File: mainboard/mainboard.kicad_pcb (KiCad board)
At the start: 2 copper layers, 50 x 99.1 mm, 93 parts, among them J1 Eurorack_Power, J2 Inv1, J3 Inv2, J4 Ver2, J5 Ver1, J6 Conn_02x04_Counter_Clockwise, J7 Conn_02x03_Counter_Clockwise, J8 Out2, J9 Out1, Q1 BC557, Q10 BC557, Q11 BC557, Q12 BC557, Q13 BC547, Q14 BC547, Q15 BC557, Q16 BC557, Q17 BC547, Q18 BC547, Q19 BC557, Q2 BC557, Q20 BC557, Q21 BC547, Q22 BC547, Q23 BC557, Q24 BC547, Q25 BC547, Q3 BC547, Q4 BC547, Q5 BC547, Q6 BC547, Q7 BC547, Q8 BC547, Q9 BC557, U1 L78L09_TO92, U2 TL074

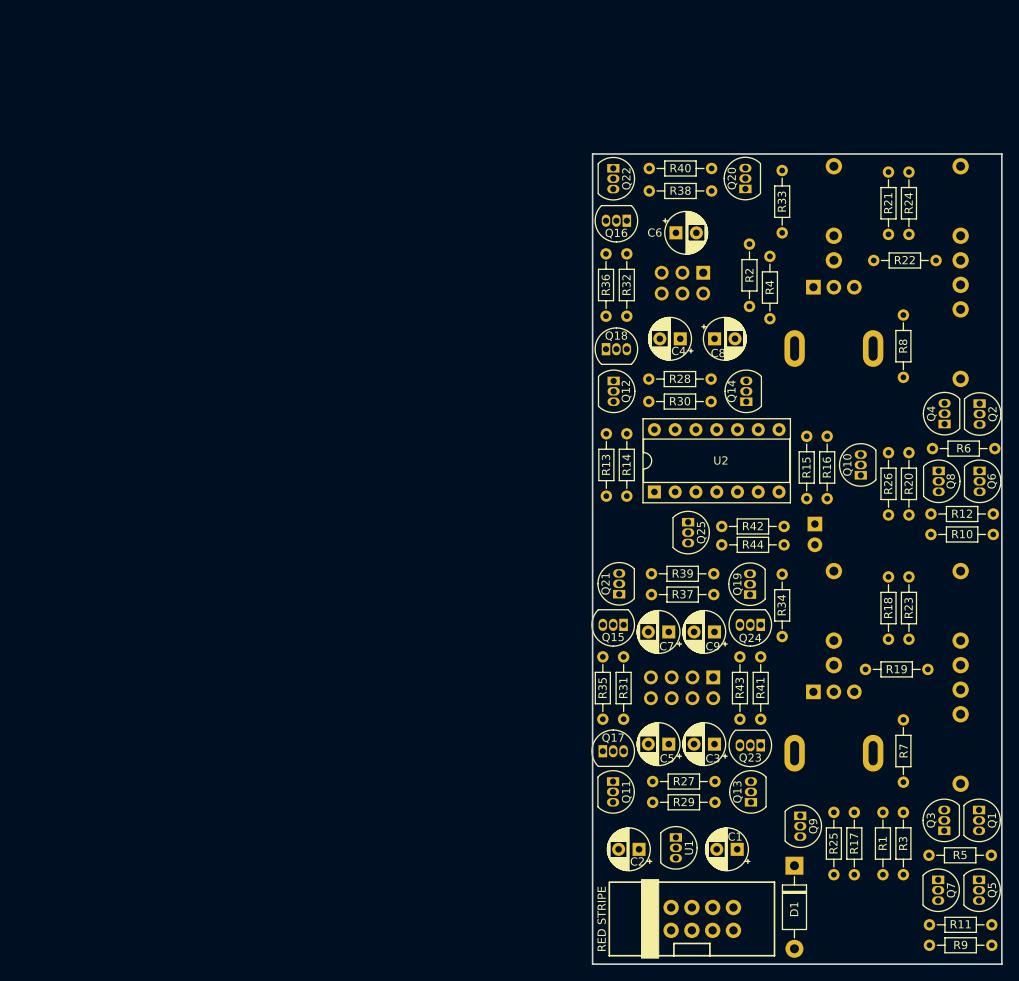
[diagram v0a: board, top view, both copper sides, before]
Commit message: Routing
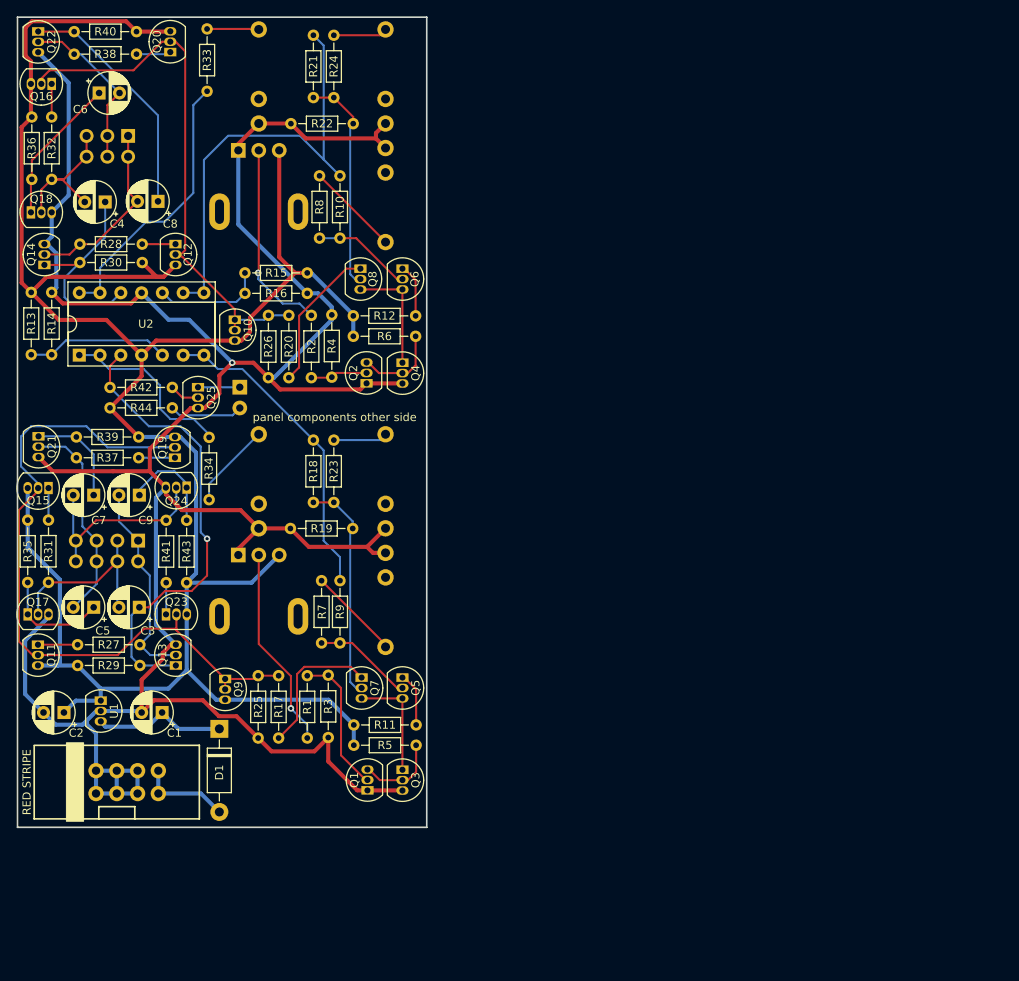
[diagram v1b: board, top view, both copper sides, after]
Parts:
- moved Q14 87.4 mm to (16.8, 44.0)
- moved R9 84.8 mm to (52.9, 82.7), turned to -90 degrees
- moved R10 84.5 mm to (52.9, 33.1), turned to -90 degrees
- moved R30 79.0 mm to (21.1, 43.8), turned to 0 degrees
- moved R28 78.9 mm to (21.1, 41.5), turned to 0 degrees
- moved Q10 78.9 mm to (40.1, 50.8), turned to -90 degrees
- moved R44 76.7 mm to (24.8, 61.5)
- moved R20 76.4 mm to (46.7, 57.8), turned to 90 degrees
- moved R26 76.4 mm to (44.2, 57.8), turned to 90 degrees
- moved R16 75.5 mm to (41.3, 47.5), turned to 0 degrees
- moved Q2 75.0 mm to (56.2, 58.5), turned to 90 degrees
- moved Q8 74.9 mm to (55.4, 44.5)
- moved Q1 74.8 mm to (56.3, 108.3), turned to 90 degrees
- moved Q6 74.8 mm to (60.6, 44.5)
- moved Q5 74.7 mm to (60.6, 94.5)
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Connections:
- U2 pad 1: MIDO1 -> Net-(R34-Pad2)
- U2 pad 10: Net-(C4-Pad1) -> Net-(R15-Pad2)
- U2 pad 12: Net-(R15-Pad2) -> Net-(C4-Pad1)
- U2 pad 13: MIDO2 -> Net-(R33-Pad2)
- U2 pad 14: MIDO2 -> Net-(R33-Pad2)
- U2 pad 2: MIDO1 -> Net-(R34-Pad2)
- U2 pad 3: Net-(R13-Pad2) -> Out1
- U2 pad 5: Out1 -> Net-(R13-Pad2)
- U2 pad 6: Net-(R34-Pad2) -> MIDO1
- U2 pad 7: Net-(R34-Pad2) -> MIDO1
- U2 pad 8: Net-(R33-Pad2) -> MIDO2
- U2 pad 9: Net-(R33-Pad2) -> MIDO2
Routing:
- net GND: track 0.00 -> 340.3 mm, vias 0 -> 1
- net +9V: track 0.00 -> 281.1 mm
- net Net-(Q11-Pad2): track 0.00 -> 86.9 mm
- net Net-(Q10-Pad1): track 0.00 -> 65.7 mm
- net Out1: track 0.00 -> 56.9 mm, vias 0 -> 1
- net MIDO2: track 0.00 -> 54.4 mm
- net MIDO1: track 0.00 -> 38.8 mm
- net Net-(R33-Pad2): track 0.00 -> 33.9 mm
- net Net-(C8-Pad1): track 0.00 -> 29.4 mm
- net Net-(Q7-Pad2): track 0.00 -> 27.2 mm
- net Net-(Q8-Pad2): track 0.00 -> 26.7 mm
- net Net-(C4-Pad1): track 0.00 -> 25.8 mm
- net N3: track 0.00 -> 25.7 mm
- net N1: track 0.00 -> 25.3 mm
- net Net-(R1-Pad1): track 0.00 -> 24.8 mm, vias 0 -> 1
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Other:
- board text added: "panel components other side"
- board text added: "panel components this side"
- board text added: "pcb by Neil Massey from a circuit by Ciat-Lonbarde thanks to Josh Rodriguez"
